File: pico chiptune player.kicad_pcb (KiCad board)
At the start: 4 copper layers, 80 x 70.8 mm, 31 parts, among them J1 Speaker Out, J2 MicroSD, SW1 Play / Pause, SW2 Next, SW3 Previous, U1 AY-3-8910, U2 0.96"OLED_I2C, U3 PAM8302AAS

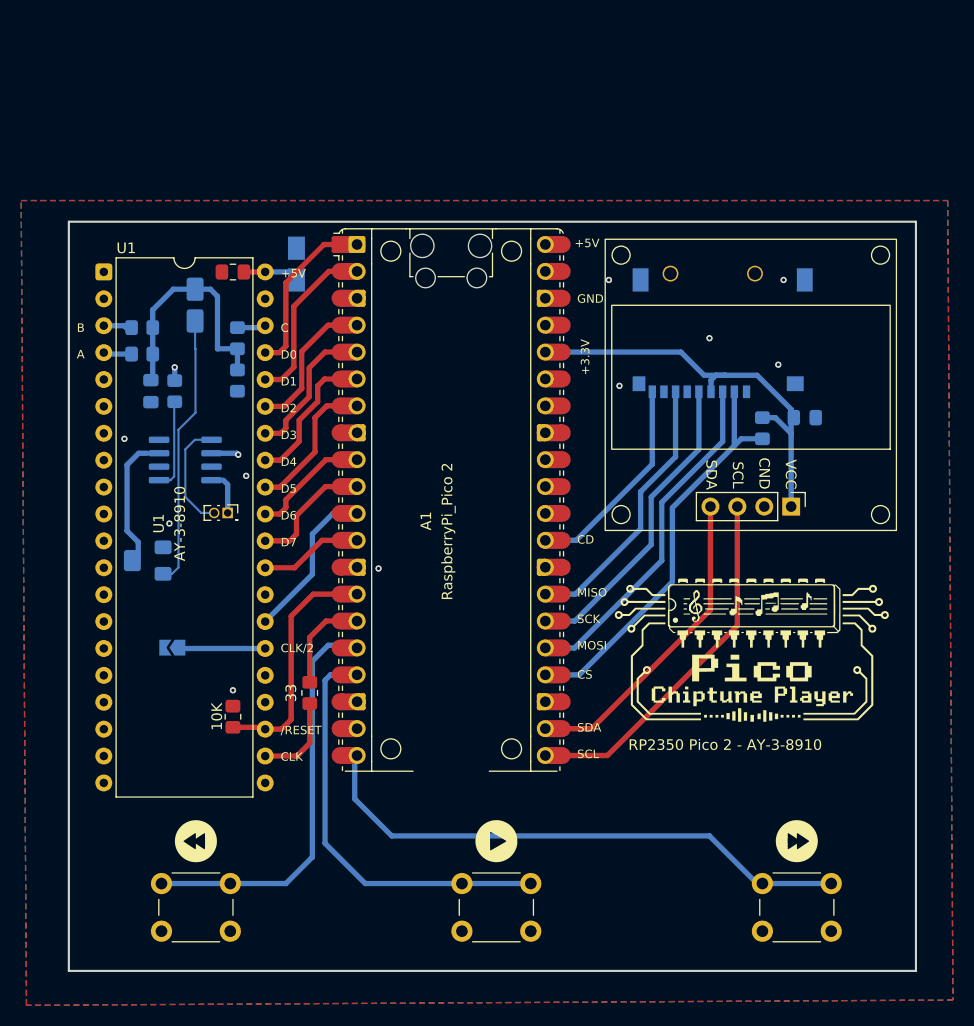
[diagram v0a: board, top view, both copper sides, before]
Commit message: Refactor code structure for improved readability and maintainability
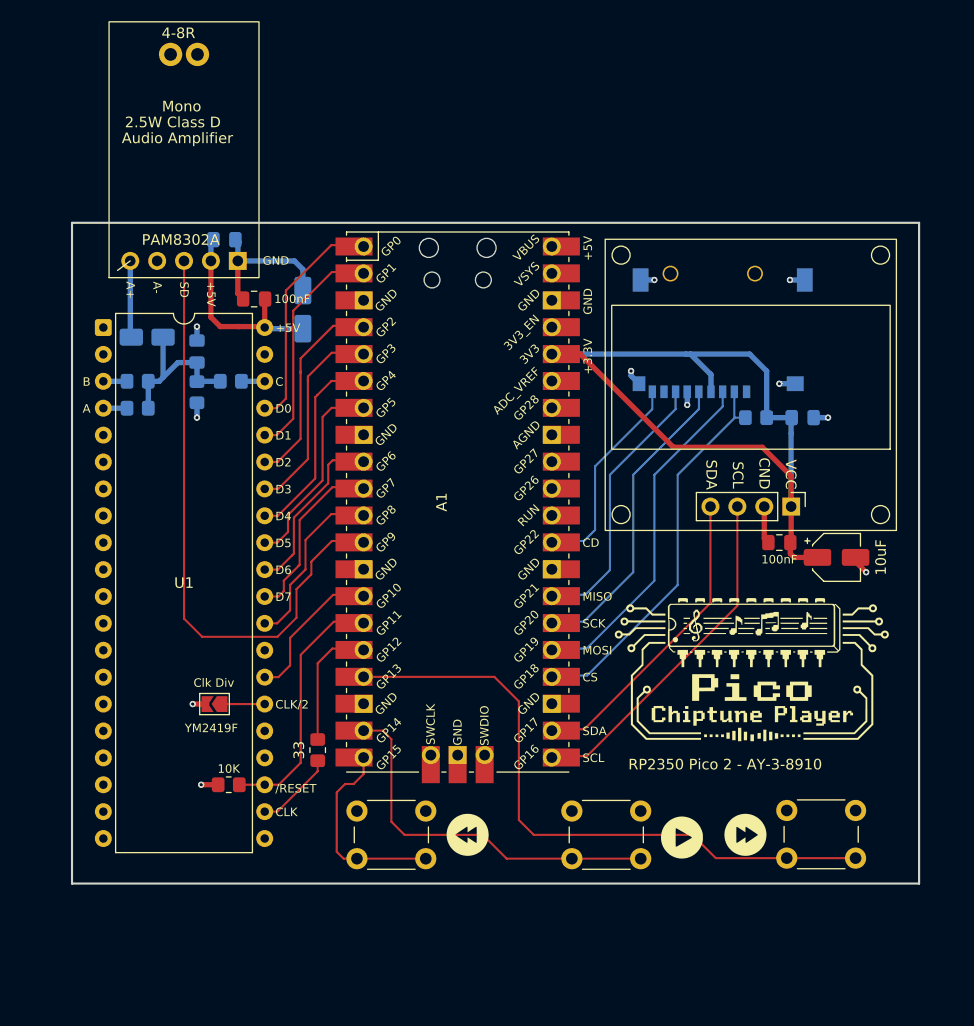
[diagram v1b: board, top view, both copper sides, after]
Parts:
- removed J1: Speaker Out, Connector_PinSocket_1.27mm:PinSocket_2x01_P1.27mm_Vertical
- removed R6: 10K, Resistor_SMD:R_0805_2012Metric_Pad1.20x1.40mm_HandSolder
- removed RV1: 3224W-1-103E, Potentiometer_SMD:Potentiometer_Bourns_3224W_Vertical
- added C6: 10uF, Capacitor_SMD:CP_Elec_4x5.4, F.Cu at (181.0, 104.2)
- added C7: 100nF, Capacitor_SMD:C_0805_2012Metric_Pad1.18x1.45mm_HandSolder, F.Cu at (175.6, 102.8)
- added C8: 100nF, Capacitor_SMD:C_0805_2012Metric_Pad1.18x1.45mm_HandSolder, B.Cu at (123.2, 74.2)
- added G***: LOGO, LOGO, B.Cu at (173.0, 107.4)
- A1: footprint Module_RaspberryPi_Pico:RaspberryPi_Pico_Common -> TMCu Module:RPi_Pico_SMD_TH
- C1: footprint Capacitor_SMD:CP_Elec_3x5.3 -> Capacitor_SMD:CP_Elec_4x5.4
- C4, C5: value 10nF -> 100nF
- J2: footprint terence:MicroSD -> Terence:MicroSD
- JP1: moved to F.Cu
- U2: footprint terence:0.96OLED I2C -> TModules:OLED 0.96 I2C
- U3: value PAM8302AAS -> PAM8302; footprint Package_SO:SOIC-8_3.9x4.9mm_P1.27mm -> TModules:PAM8302A_Module; moved to F.Cu
- moved U3 29.3 mm to (119.4, 65.7)
- moved G*** 25.7 mm to (146.2, 130.4)
- moved SW3 25.1 mm to (142.2, 132.7), turned to 180 degrees
- moved G*** 19.9 mm to (139.0, 130.4)
- moved G*** 17.5 mm to (166.4, 130.7)
- moved SW1 17.0 mm to (162.5, 132.7), turned to 180 degrees
- moved G*** 12.4 mm to (159.3, 130.4), turned to 0 degrees
- moved SW2 9.12 mm to (182.8, 132.6), turned to 180 degrees
- moved G*** 7.28 mm to (179.6, 130.3)
- moved JP1 6.65 mm to (122.3, 118.0)
- moved R3 6.43 mm to (123.6, 125.7), turned to 180 degrees
- moved C4 5.74 mm to (120.6, 84.8), turned to 90 degrees
- moved R2 5.45 mm to (132.0, 122.4)
- moved C3 5.44 mm to (115.9, 83.4), turned to 180 degrees
- moved U1 5.25 mm to (111.8, 82.5)
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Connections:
- A1 pad 11: /BDIR -> /BC1
- A1 pad 12: /BC1 -> /SD_Amp
- A1 pad 14: /~{RESET} -> /BDIR
- A1 pad 15: Net-(A1-GPIO11) -> /~{RESET}
- A1 pad 16: /SW_PREV -> Net-(A1-GPIO12)
- A1 pad 17: /SW_PLAY -> /SW_NEXT
- A1 pad 19: unconnected-(A1-GPIO14-Pad19) -> /SW_PLAY
- A1 pad 20: /SW_NEXT -> /SW_PREV
- C3 pad 2: Net-(C3-Pad2) -> Net-(U3-A+)
- R2 pad 2: Net-(R2-Pad2) -> Net-(A1-GPIO12)
- U3 pad 1: Net-(U3-~{SD}) -> GND
- U3 pad 2: unconnected-(U3-NC-Pad2) -> +5V
- U3 pad 3: Net-(U3-IN+) -> /SD_Amp
- U3 pad 5: Net-(J1-Pin_2) -> Net-(U3-A+)
- U3 pad 6: +5V -> unconnected-(U3-OUT+-Pad6)
- U3 pad 7: GND -> unconnected-(U3-OUT--Pad7)
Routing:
- net /SD_Amp: track 0.00 -> 56.9 mm
- net +3.3V: track 40.6 -> 78.9 mm
- net GND: track 0.63 -> 34.6 mm, vias 10 -> 11
- net Net-(C3-Pad2): track 25.7 -> 0.00 mm
- net /SW_PREV: track 38.7 -> 19.1 mm
- net Net-(A1-GPIO12): track 0.00 -> 11.8 mm
- net Net-(U3-IN+): track 11.8 -> 0.00 mm
- net +5V: track 9.11 -> 20.5 mm, vias 2 -> 0
- net Net-(J1-Pin_2): track 10.7 -> 0.00 mm
- net Net-(A1-GPIO11): track 9.36 -> 0.00 mm
- net Net-(U3-~{SD}): track 8.64 -> 0.00 mm
- net /SW_NEXT: track 52.5 -> 60.1 mm
- net Net-(U3-A+): track 0.00 -> 7.24 mm
- net Net-(C3-Pad1): track 22.8 -> 15.7 mm
- net /BC1: track 9.75 -> 16.0 mm
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- removed copper zone on B.Cu, net GND
- removed copper zone on F.Cu, net GND
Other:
- board size 80 x 70.8 mm -> 80 x 62.4 mm
- board text added: "14082026"
- board text added: "Terence Ang / MotionFxDesign"
- board text added: "YM2149F"
- board text added: "YM2419F"
- board text added: "https://github.com/terenceang/pico-chiptune-player"
- board text removed: "Terence Ang / MotionFxDesign 2026"
- board text removed: "VOL"
